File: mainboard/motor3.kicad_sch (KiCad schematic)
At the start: 12 parts, among them U3 DRV8323RSRGZT

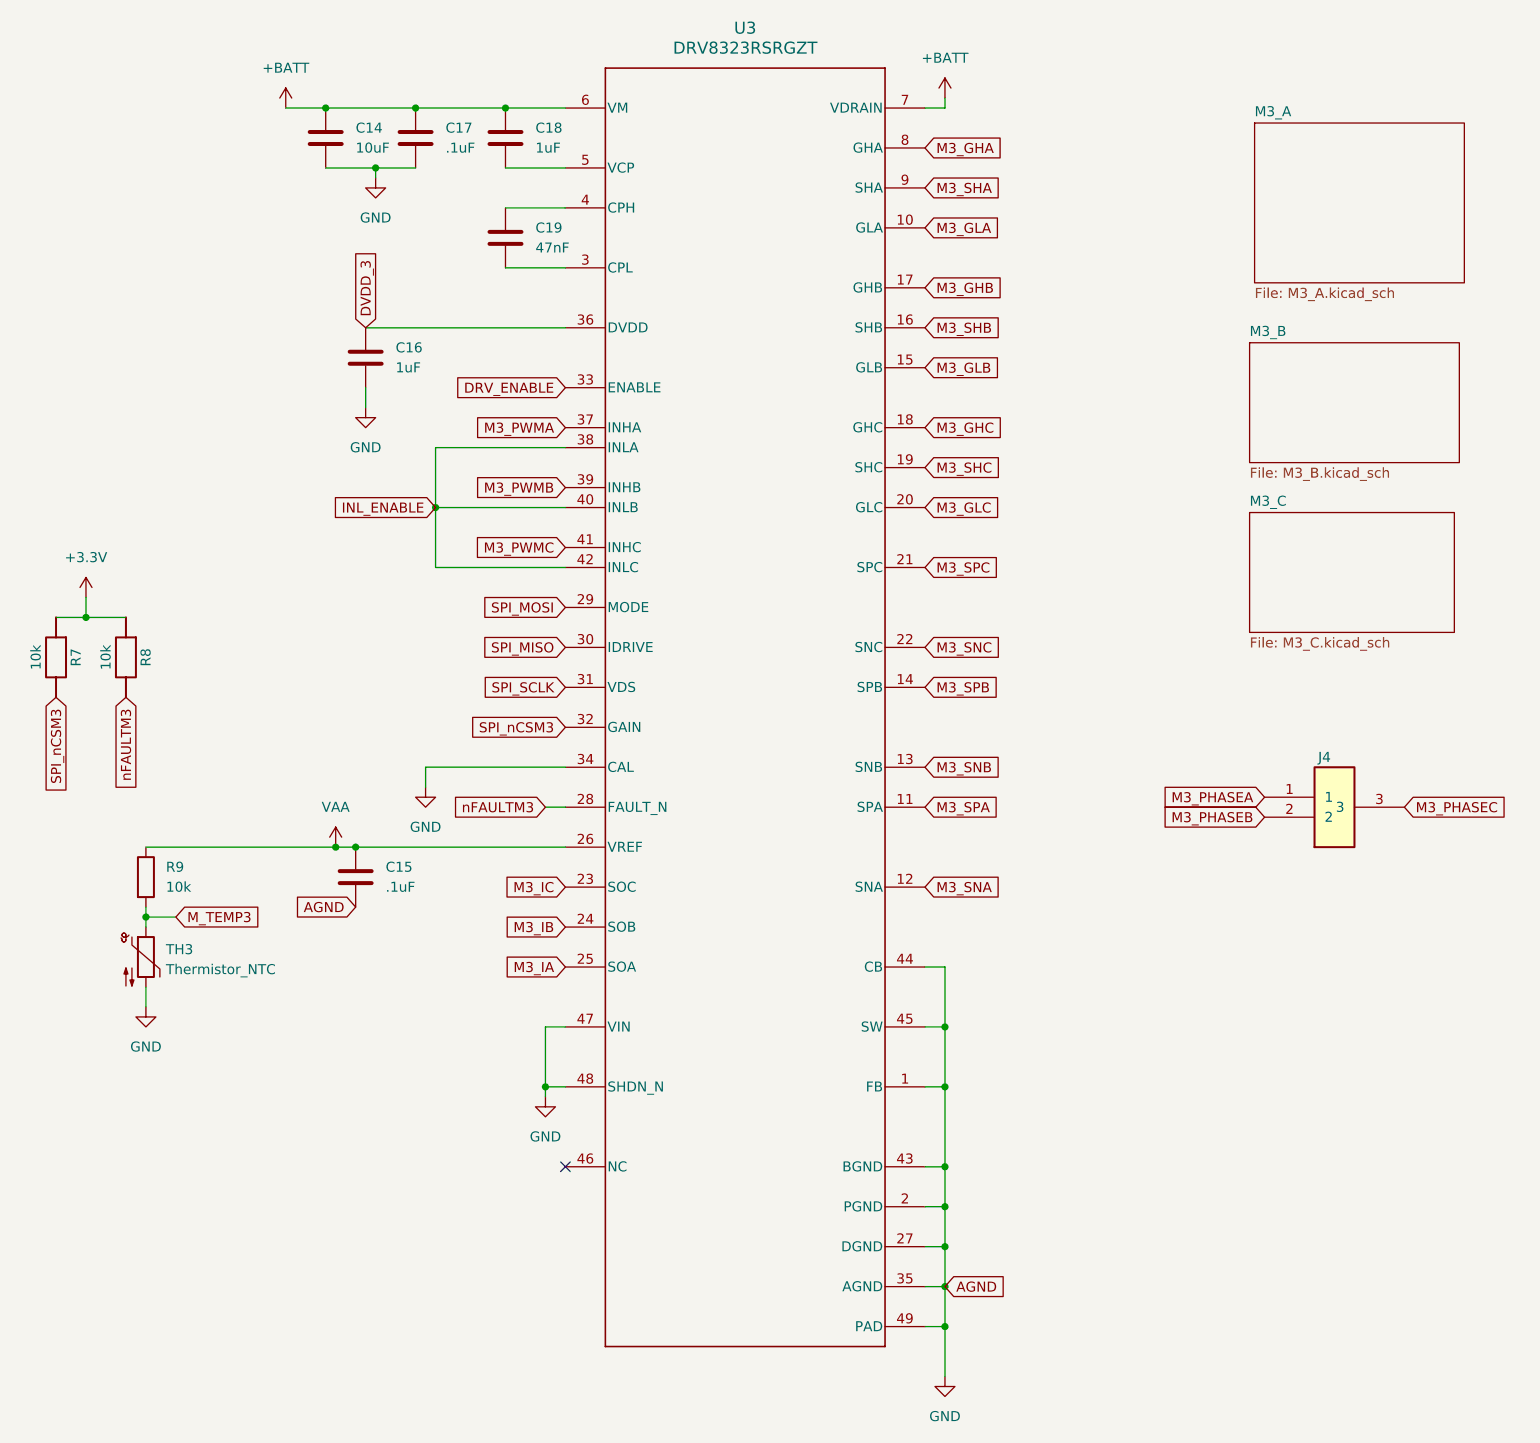
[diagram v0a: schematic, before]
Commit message: Initial layout completed
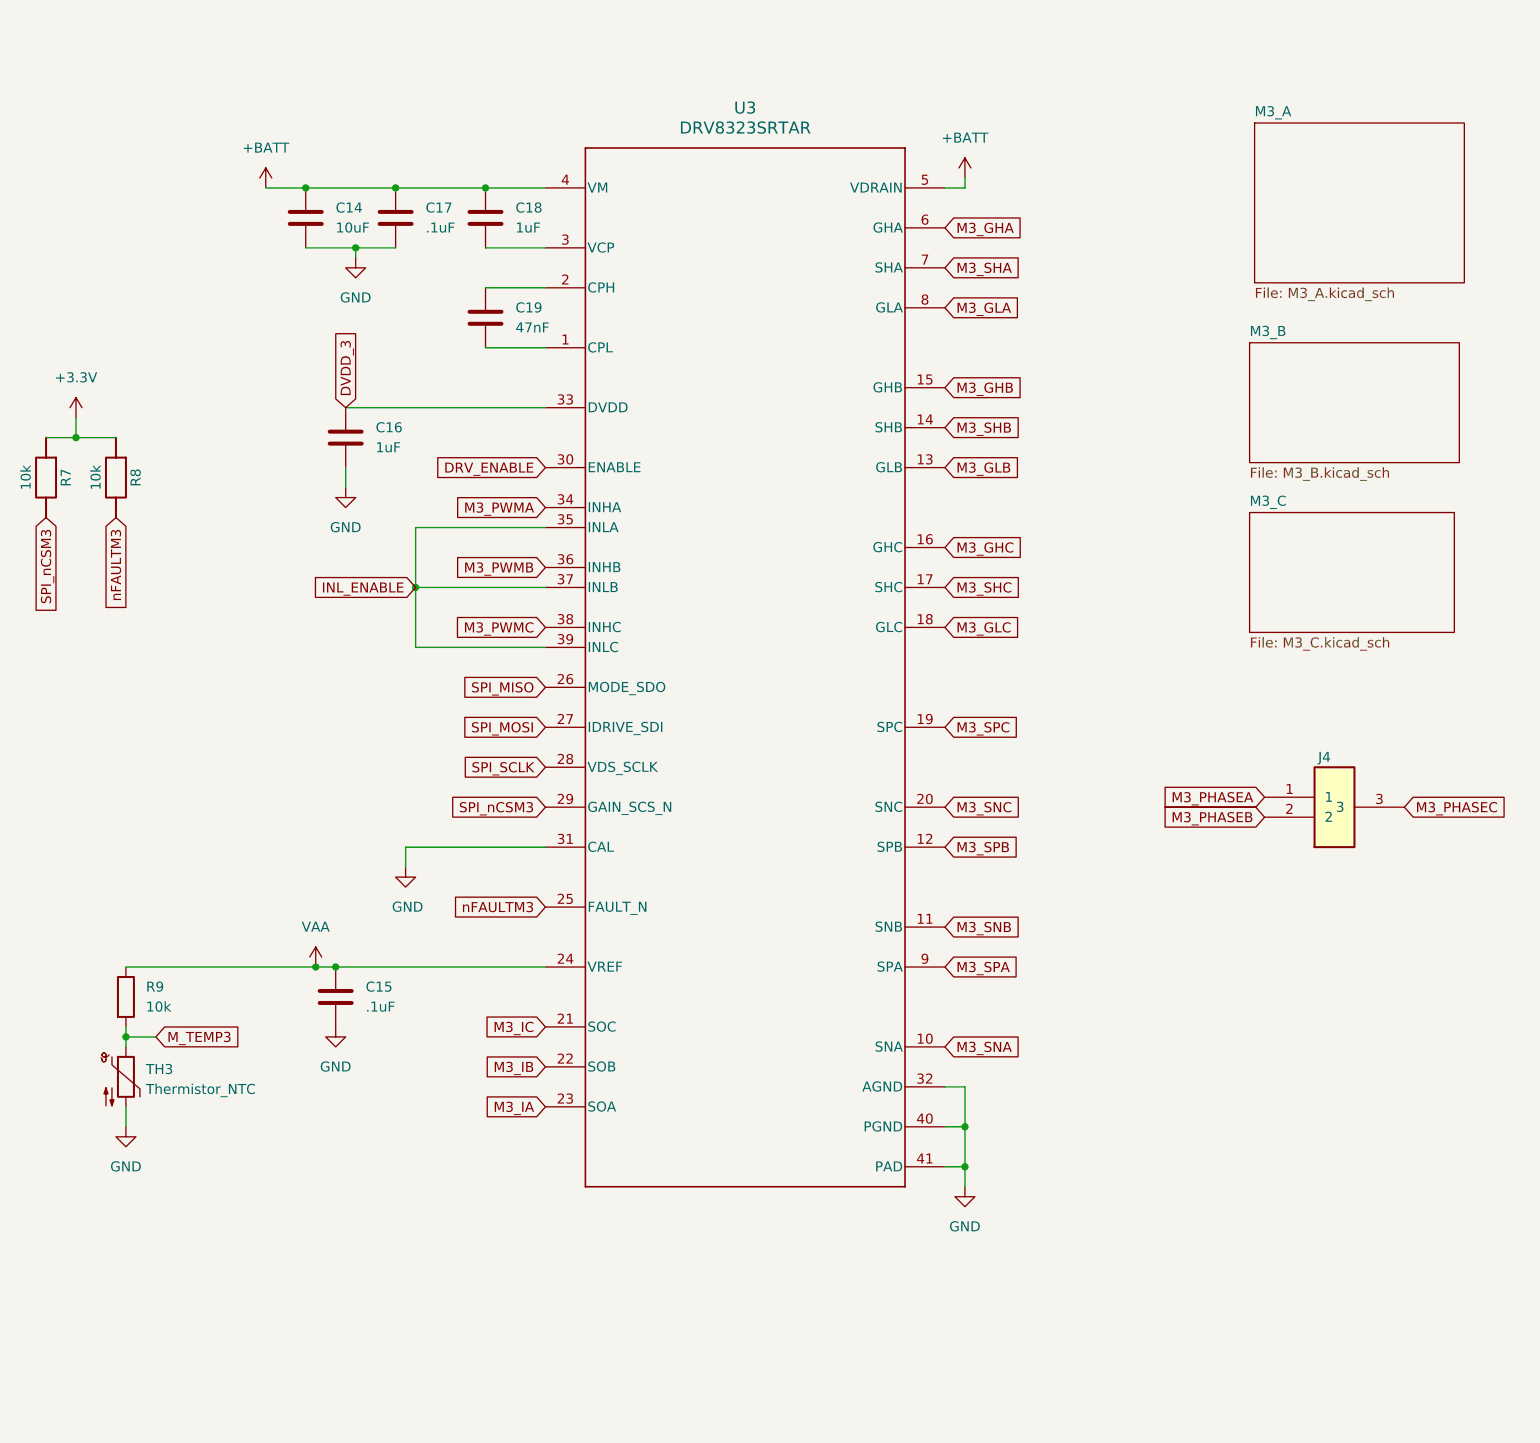
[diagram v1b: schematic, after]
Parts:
- removed U3: DRV8323RSRGZT, DRV8323RSRGZT_new:RGZ0048A, symbol DRV8323RSRGZT_new:DRV8323RSRGZT
- added U3: DRV8323SRTAR, DRV8323SRTAR:RTA0040B_NV, symbol DRV8323SR:DRV8323SRTAR
- C14: footprint Capacitor_SMD:C_1210_3225Metric -> Capacitor_SMD:C_1206_3216Metric
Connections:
- net +BATT: now also U3.4 (VM), U3.5 (VDRAIN)
- net DRV_ENABLE: now also U3.30 (ENABLE)
- net DVDD_3: now also U3.33 (DVDD)
- net GND: now also U3.31 (CAL), U3.32 (AGND), U3.40 (PGND), U3.41 (PAD)
- net INL_ENABLE: now also U3.35 (INLA), U3.37 (INLB), U3.39 (INLC)
- net M3_GHA: now also U3.6 (GHA)
- net M3_GHB: now also U3.15 (GHB)
- net M3_GHC: now also U3.16 (GHC)
- net M3_GLA: now also U3.8 (GLA)
- net M3_GLB: now also U3.13 (GLB)
- net M3_GLC: now also U3.18 (GLC)
- net M3_IA: now also U3.23 (SOA)
- net M3_IB: now also U3.22 (SOB)
- net M3_IC: now also U3.21 (SOC)
- net M3_PWMA: now also U3.34 (INHA)
- net M3_PWMB: now also U3.36 (INHB)
- net M3_PWMC: now also U3.38 (INHC)
- net M3_SHA: now also U3.7 (SHA)
- net M3_SHB: now also U3.14 (SHB)
- net M3_SHC: now also U3.17 (SHC)
- net M3_SNA: now also U3.10 (SNA)
- net M3_SNB: now also U3.11 (SNB)
- net M3_SNC: now also U3.20 (SNC)
- net M3_SPA: now also U3.9 (SPA)
- net M3_SPB: now also U3.12 (SPB)
- net M3_SPC: now also U3.19 (SPC)
- net SPI_MISO: now also U3.26 (MODE_SDO)
- net SPI_MOSI: now also U3.27 (IDRIVE_SDI)
- net SPI_SCLK: now also U3.28 (VDS_SCLK)
- net SPI_nCSM3: now also U3.29 (GAIN_SCS_N)
- net VAA: now also U3.24 (VREF)
- net nFAULTM3: now also U3.25 (FAULT_N)
- net at C18.2: now also U3.3 (VCP)
- net at C19.1: now also U3.2 (CPH)
- net at C19.2: now also U3.1 (CPL)
- no-connect marks 1 -> 0
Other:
- moved on the sheet: C14, C15, C16, C17, C18, C19, R7, R8, R9, TH3
